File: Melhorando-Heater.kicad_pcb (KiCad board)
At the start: 2 copper layers, 48.5 x 41.4 mm, 23 parts, among them J1 Conn_01x04, J2 1x03, J3 1x04, Q1 BC817, U1 MSP430FR2433IRGET

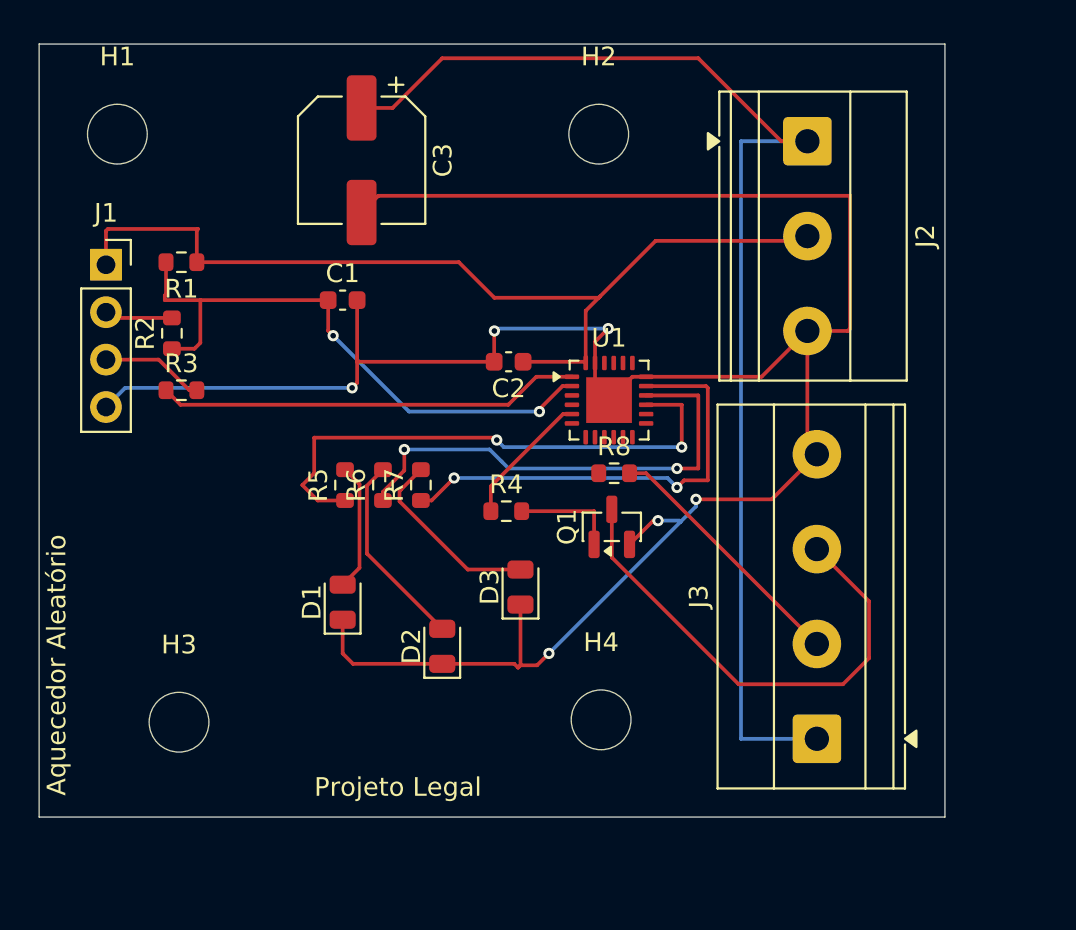
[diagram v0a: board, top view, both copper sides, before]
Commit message: :minidisc: delivered finished board
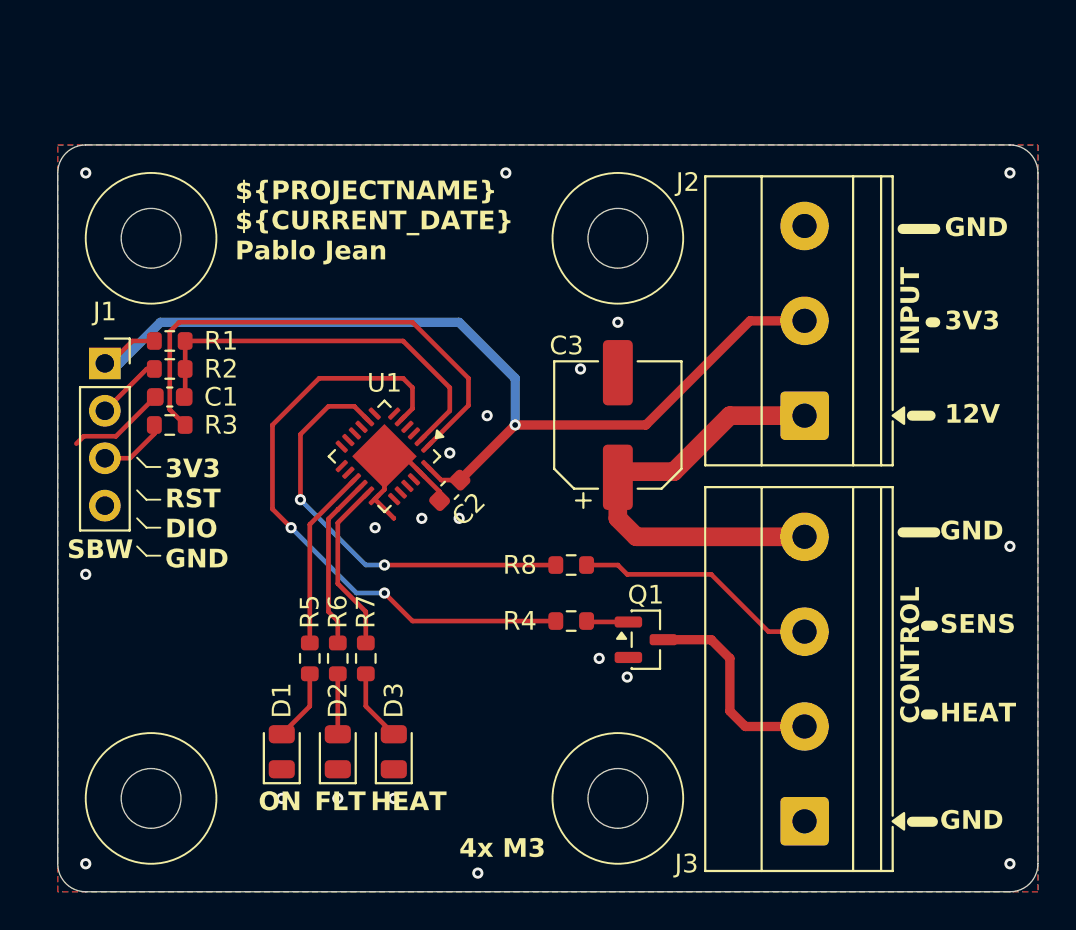
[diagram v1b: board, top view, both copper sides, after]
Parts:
- moved C3 19.7 mm to (190.0, 90.0), turned to 90 degrees
- moved J2 14.7 mm to (200.0, 89.5), turned to 90 degrees
- moved U1 12.4 mm to (177.5, 91.7), turned to -135 degrees
- moved D3 11.1 mm to (178.0, 107.5)
- moved C1 10.6 mm to (166.0, 88.5), turned to 180 degrees
- moved R7 9.74 mm to (176.5, 102.5), turned to -90 degrees
- moved R6 9.59 mm to (175.0, 102.5), turned to -90 degrees
- moved R5 9.47 mm to (173.5, 102.5), turned to -90 degrees
- moved D1 8.65 mm to (172.0, 107.5)
- moved D2 7.95 mm to (175.0, 107.5)
- moved C2 7.57 mm to (181.0, 93.5), turned to -135 degrees
- moved R4 6.84 mm to (187.5, 100.5)
- moved Q1 6.31 mm to (191.5, 101.5), turned to 0 degrees
- moved H1 5.86 mm to (165.0, 80.0)
- moved H2 5.67 mm to (190.0, 80.0)
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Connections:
- J3 pad 1: 12V -> GND
- J3 pad 2: /P_SENSOR -> /P_HEATER
- J3 pad 3: /P_HEATER -> /P_SENSOR
- J3 pad 4: GND -> 12V
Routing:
- net GND: track 132.0 -> 13.4 mm, vias 6 -> 20
- net 12V: track 66.4 -> 24.0 mm
- net /M_HEATER: track 7.28 -> 32.9 mm, vias 0 -> 2
- net /S_SENSOR: track 0.00 -> 23.2 mm, vias 0 -> 2
- net /LED_ON: track 29.5 -> 9.77 mm, vias 2 -> 0
- net /LED_FAULT: track 26.1 -> 9.38 mm, vias 2 -> 0
- net /P_HEATER: track 26.7 -> 11.1 mm
- net /LED_HEAT: track 24.5 -> 9.35 mm, vias 2 -> 0
- net /MCU_RST: track 31.9 -> 21.7 mm, vias 2 -> 0
- net Net-(D2-A): track 10.5 -> 3.24 mm
- net Net-(D3-A): track 10.2 -> 3.86 mm
- net /MCU_DIO: track 22.7 -> 27.4 mm
- net Net-(Q1-B): track 5.65 -> 2.26 mm
- net 3V3: track 50.7 -> 53.8 mm, vias 0 -> 1
- net Net-(D1-A): track 6.85 -> 3.86 mm
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- added copper zone on B.Cu, net GND
- added copper zone on F.Cu, net GND
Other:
- board size 48.5 x 41.4 mm -> 52.5 x 40 mm
- board text added: "${PROJECTNAME} ${CURRENT_DATE} Pablo Jean"
- board text added: "12V"
- board text added: "3V3"
- board text added: "3V3 RST DIO GND"
- board text added: "4x M3"
- board text added: "CONTROL"
- board text added: "FLT"
- board text added: "GND"
- board text added: "HEAT"
- board text added: "INPUT"
- board text added: "ON"
- board text added: "SBW"
- board text added: "SENS"
- board text removed: "Aquecedor Aleatório"
- board text removed: "Projeto Legal"
